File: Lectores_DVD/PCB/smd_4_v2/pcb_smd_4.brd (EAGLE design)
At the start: 20.8 x 22.8 mm, 2 parts, among them J1 52793-0470

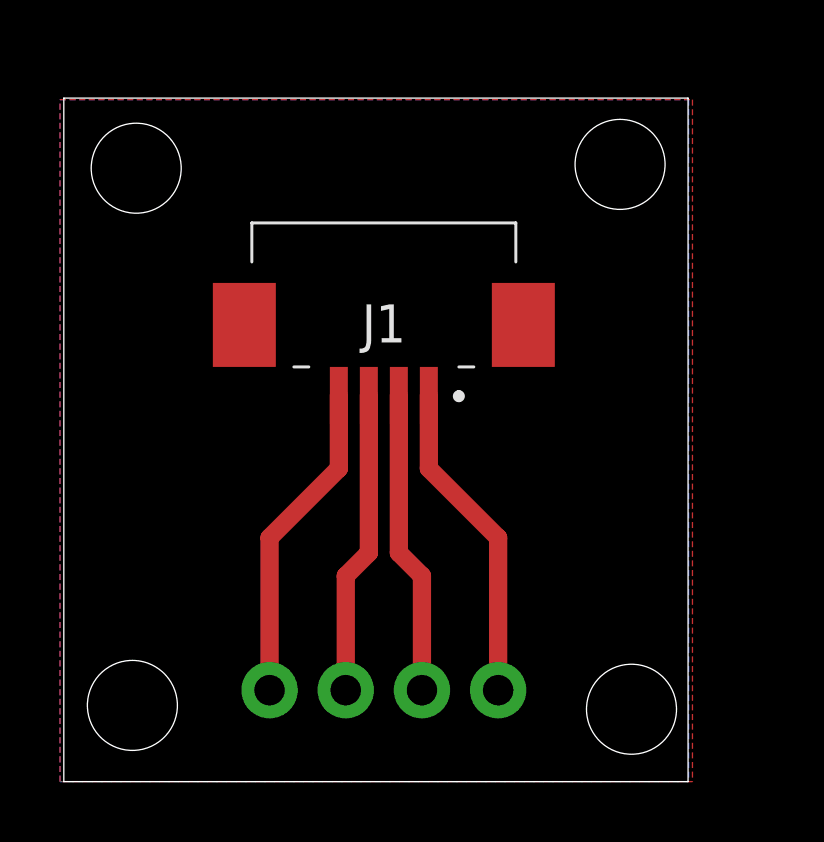
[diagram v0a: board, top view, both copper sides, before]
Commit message: Actualizacion
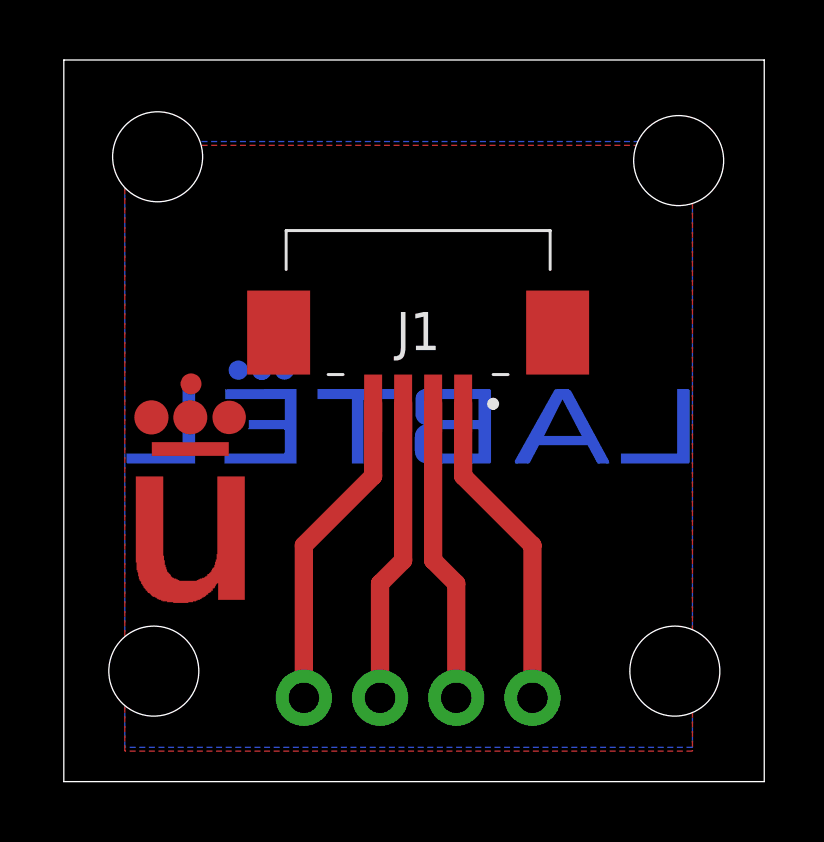
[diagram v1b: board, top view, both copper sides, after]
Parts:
- added U$1: (no value), logos_top:URJC
- added U$2: (no value), logos_top:LABTEL
- moved J1 1.17 mm to (13.8, 16.3)
- moved J2 1.17 mm to (17.7, 3.56)
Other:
- board size 20.8 x 22.8 mm -> 23.3 x 24.1 mm
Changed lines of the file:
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@@
 <setting verticaltext="up"/>
 </settings>
-<grid distance="1.27" unitdist="mm" unit="mm" style="lines" multiple="1" display="no" altdistance="5" altunitdist="mil" altunit="mm"/>
+<grid distance="0.127" unitdist="mm" unit="mm" style="lines" multiple="1" display="no" altdistance="5" altunitdist="mil" altunit="mm"/>
 <layers>
 <layer number="1" name="Top" color="4" fill="1" visible="yes" active="yes"/>
@@
 <board>
 <plain>
-<wire x1="2.032" y1="0.762" x2="22.84" y2="0.762" width="0" layer="20"/>
-<wire x1="22.84" y1="0.762" x2="22.84" y2="23.546" width="0" layer="20"/>
-<wire x1="22.84" y1="23.546" x2="2.032" y2="23.546" width="0" layer="20"/>
-<wire x1="2.032" y1="23.546" x2="2.032" y2="0.762" width="0" layer="20"/>
-<hole x="4.445" y="21.209" drill="3"/>
-<hole x="20.574" y="21.336" drill="3"/>
-<hole x="20.955" y="3.175" drill="3"/>
-<hole x="4.318" y="3.302" drill="3"/>
+<wire x1="2.032" y1="0.762" x2="25.38" y2="0.762" width="0" layer="20"/>
+<wire x1="25.38" y1="0.762" x2="25.38" y2="24.816" width="0" layer="20"/>
+<wire x1="25.38" y1="24.816" x2="2.032" y2="24.816" width="0" layer="20"/>
+<wire x1="2.032" y1="24.816" x2="2.032" y2="0.762" width="0" layer="20"/>
+<hole x="5.159" y="21.59" drill="3"/>
+<hole x="22.527" y="21.463" drill="3"/>
+<hole x="22.4" y="4.445" drill="3"/>
+<hole x="5.032" y="4.445" drill="3"/>
 </plain>
 <attributes>
@@
 </autorouter>
 <elements>
-<element name="J1" library="52793-0470" package="527930472" value="52793-0470" x="12.7" y="16.51" smashed="yes" rot="R180">
-<attribute name="ALLIED_NUMBER" value="71463721" x="-6.35" y="20.32" size="1.778" layer="27" rot="R180" display="off"/>
-<attribute name="ALLIED_PRICE-STOCK" value="https://www.alliedelec.com/molexincorporated-52793-0470/71463721/" x="-6.35" y="20.32" size="1.778" layer="27" rot="R180" display="off"/>
-<attribute name="DESCRIPTION" value="Molex 52793 Series 1mm Pitch 4 Way SMT Female FPC Connector, Non-ZIF" x="-6.35" y="20.32" size="1.778" layer="27" rot="R180" display="off"/>
-<attribute name="HEIGHT" value="3.1mm" x="-6.35" y="20.32" size="1.778" layer="27" rot="R180" display="off"/>
-<attribute name="MANUFACTURER_NAME" value="Molex" x="-6.35" y="20.32" size="1.778" layer="27" rot="R180" display="off"/>
-<attribute name="MANUFACTURER_PART_NUMBER" value="52793-0470" x="-6.35" y="20.32" size="1.778" layer="27" rot="R180" display="off"/>
-<attribute name="MOUSER_PART_NUMBER" value="538-52793-0470" x="-6.35" y="20.32" size="1.778" layer="27" rot="R180" display="off"/>
-<attribute name="MOUSER_PRICE-STOCK" value="https://www.mouser.com/Search/Refine.aspx?Keyword=538-52793-0470" x="-6.35" y="20.32" size="1.778" layer="27" rot="R180" display="off"/>
-<attribute name="NAME" x="12.7" y="16.035" size="1.27" layer="25" rot="R180" align="center"/>
-<attribute name="RS_PART_NUMBER" value="1791963" x="-6.35" y="20.32" size="1.778" layer="27" rot="R180" display="off"/>
-<attribute name="RS_PRICE-STOCK" value="http://uk.rs-online.com/web/p/products/1791963" x="-6.35" y="20.32" size="1.778" layer="27" rot="R180" display="off"/>
-<attribute name="VALUE" x="12.7" y="16.035" size="1.27" layer="27" rot="R180" align="center"/>
+<element name="J1" library="52793-0470" package="527930472" value="52793-0470" x="13.843" y="16.256" smashed="yes" rot="R180">
+<attribute name="ALLIED_NUMBER" value="71463721" x="-5.207" y="20.066" size="1.778" layer="27" rot="R180" display="off"/>
+<attribute name="ALLIED_PRICE-STOCK" value="https://www.alliedelec.com/molexincorporated-52793-0470/71463721/" x="-5.207" y="20.066" size="1.778" layer="27" rot="R180" display="off"/>
+<attribute name="DESCRIPTION" value="Molex 52793 Series 1mm Pitch 4 Way SMT Female FPC Connector, Non-ZIF" x="-5.207" y="20.066" size="1.778" layer="27" rot="R180" display="off"/>
+<attribute name="HEIGHT" value="3.1mm" x="-5.207" y="20.066" size="1.778" layer="27" rot="R180" display="off"/>
+<attribute name="MANUFACTURER_NAME" value="Molex" x="-5.207" y="20.066" size="1.778" layer="27" rot="R180" display="off"/>
+<attribute name="MANUFACTURER_PART_NUMBER" value="52793-0470" x="-5.207" y="20.066" size="1.778" layer="27" rot="R180" display="off"/>
+<attribute name="MOUSER_PART_NUMBER" value="538-52793-0470" x="-5.207" y="20.066" size="1.778" layer="27" rot="R180" display="off"/>
+<attribute name="MOUSER_PRICE-STOCK" value="https://www.mouser.com/Search/Refine.aspx?Keyword=538-52793-0470" x="-5.207" y="20.066" size="1.778" layer="27" rot="R180" display="off"/>
+<attribute name="NAME" x="13.843" y="15.781" size="1.27" layer="25" rot="R180" align="center"/>
+<attribute name="RS_PART_NUMBER" value="1791963" x="-5.207" y="20.066" size="1.778" layer="27" rot="R180" display="off"/>
+<attribute name="RS_PRICE-STOCK" value="http://uk.rs-online.com/web/p/products/1791963" x="-5.207" y="20.066" size="1.778" layer="27" rot="R180" display="off"/>
+<attribute name="VALUE" x="13.843" y="15.781" size="1.27" layer="27" rot="R180" align="center"/>
 </element>
-<element name="J2" library="SparkFun-Connectors" package="1X04" value="" x="16.51" y="3.81" smashed="yes" rot="MR0">
-<attribute name="NAME" x="17.78" y="5.207" size="0.6096" layer="26" font="vector" ratio="20" rot="MR0"/>
-<attribute name="PROD_ID" value="CONN-09696" x="-6.35" y="-6.35" size="1.778" layer="28" rot="MR0" display="off"/>
-<attribute name="VALUE" x="17.78" y="1.778" size="0.6096" layer="28" font="vector" ratio="20" rot="MR0"/>
+<element name="J2" library="SparkFun-Connectors" package="1X04" value="" x="17.653" y="3.556" smashed="yes" rot="MR0">
+<attribute name="NAME" x="18.923" y="4.953" size="0.6096" layer="26" font="vector" ratio="20" rot="MR0"/>
+<attribute name="PROD_ID" value="CONN-09696" x="-5.207" y="-6.604" size="1.778" layer="28" rot="MR0" display="off"/>
+<attribute name="VALUE" x="18.923" y="1.524" size="0.6096" layer="28" font="vector" ratio="20" rot="MR0"/>
 </element>
+<element name="U$1" library="logos_top" package="URJC" value="" x="4.445" y="6.731" smashed="yes"/>
+<element name="U$2" library="logos_top" package="LABTEL" value="" x="23.495" y="10.287" smashed="yes" rot="MR0"/>
 </elements>
 <signals>
@@
 <contactref element="J1" pad="3"/>
 <contactref element="J2" pad="3"/>
-<wire x1="12.2" y1="13.635" x2="12.2" y2="8.39" width="0.6096" layer="1"/>
-<wire x1="12.2" y1="8.39" x2="11.43" y2="7.62" width="0.6096" layer="1"/>
-<wire x1="11.43" y1="7.62" x2="11.43" y2="3.81" width="0.6096" layer="1"/>
+<wire x1="13.343" y1="13.381" x2="13.343" y2="8.136" width="0.6096" layer="1"/>
+<wire x1="13.343" y1="8.136" x2="12.573" y2="7.366" width="0.6096" layer="1"/>
+<wire x1="12.573" y1="7.366" x2="12.573" y2="3.556" width="0.6096" layer="1"/>
 </signal>
 <signal name="N$5">
 <contactref element="J1" pad="1"/>
 <contactref element="J2" pad="1"/>
-<wire x1="14.2" y1="13.635" x2="14.2" y2="11.2" width="0.6096" layer="1"/>
-<wire x1="14.2" y1="11.2" x2="16.51" y2="8.89" width="0.6096" layer="1"/>
-<wire x1="16.51" y1="8.89" x2="16.51" y2="3.81" width="0.6096" layer="1"/>
+<wire x1="15.343" y1="13.381" x2="15.343" y2="10.946" width="0.6096" layer="1"/>
+<wire x1="15.343" y1="10.946" x2="17.653" y2="8.636" width="0.6096" layer="1"/>
+<wire x1="17.653" y1="8.636" x2="17.653" y2="3.556" width="0.6096" layer="1"/>
 </signal>
 <signal name="N$1">
 <contactref element="J2" pad="2"/>
 <contactref element="J1" pad="2"/>
-<wire x1="13.2" y1="13.635" x2="13.2" y2="8.39" width="0.6096" layer="1"/>
-<wire x1="13.2" y1="8.39" x2="13.97" y2="7.62" width="0.6096" layer="1"/>
-<wire x1="13.97" y1="7.62" x2="13.97" y2="3.81" width="0.6096" layer="1"/>
+<wire x1="14.343" y1="13.381" x2="14.343" y2="8.136" width="0.6096" layer="1"/>
+<wire x1="14.343" y1="8.136" x2="15.113" y2="7.366" width="0.6096" layer="1"/>
+<wire x1="15.113" y1="7.366" x2="15.113" y2="3.556" width="0.6096" layer="1"/>
 </signal>
 <signal name="N$3">
 <contactref element="J2" pad="4"/>
 <contactref element="J1" pad="4"/>
-<wire x1="11.2" y1="13.635" x2="11.2" y2="11.2" width="0.6096" layer="1"/>
-<wire x1="11.2" y1="11.2" x2="8.89" y2="8.89" width="0.6096" layer="1"/>
-<wire x1="8.89" y1="8.89" x2="8.89" y2="3.81" width="0.6096" layer="1"/>
+<wire x1="12.343" y1="13.381" x2="12.343" y2="10.946" width="0.6096" layer="1"/>
+<wire x1="12.343" y1="10.946" x2="10.033" y2="8.636" width="0.6096" layer="1"/>
+<wire x1="10.033" y1="8.636" x2="10.033" y2="3.556" width="0.6096" layer="1"/>
 </signal>
 <signal name="GND">
 <polygon width="0.1524" layer="1">
-<vertex x="1.905" y="23.495"/>
-<vertex x="22.987" y="23.495"/>
-<vertex x="22.987" y="0.762"/>
-<vertex x="1.905" y="0.762"/>
+<vertex x="4.064" y="21.971"/>
+<vertex x="22.987" y="21.971"/>
+<vertex x="22.987" y="1.778"/>
+<vertex x="4.064" y="1.778"/>
 </polygon>
 <polygon width="0.1524" layer="16">
-<vertex x="1.905" y="23.495"/>
-<vertex x="22.86" y="23.495"/>
-<vertex x="22.86" y="0.762"/>
-<vertex x="1.905" y="0.762"/>
+<vertex x="4.064" y="22.098"/>
+<vertex x="22.987" y="22.098"/>
+<vertex x="22.987" y="1.905"/>
+<vertex x="4.064" y="1.905"/>
 </polygon>
 </signal>
@@
 <mfgpreviewcolor name="substratecolor" color="0xFF786E46"/>
 </mfgpreviewcolors>
+<errors>
+</errors>
 </board>
 </drawing>
